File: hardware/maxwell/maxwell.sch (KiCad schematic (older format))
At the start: 34 parts, among them J1 Canbus 1, J2 Canbus 2, J3 Neopixel, J4 Boot Selection Jumper, J5 Charger Output, J6 Programmer, Q1 BSS138, U1 MCP2515-E/ST-SOIC, U2 SN65HVD233, U3 ITEAD_HC-05, U4 SIM800L_5-pin, U5 BOOST_BOARD, U6 TPS2511, Y1 16M

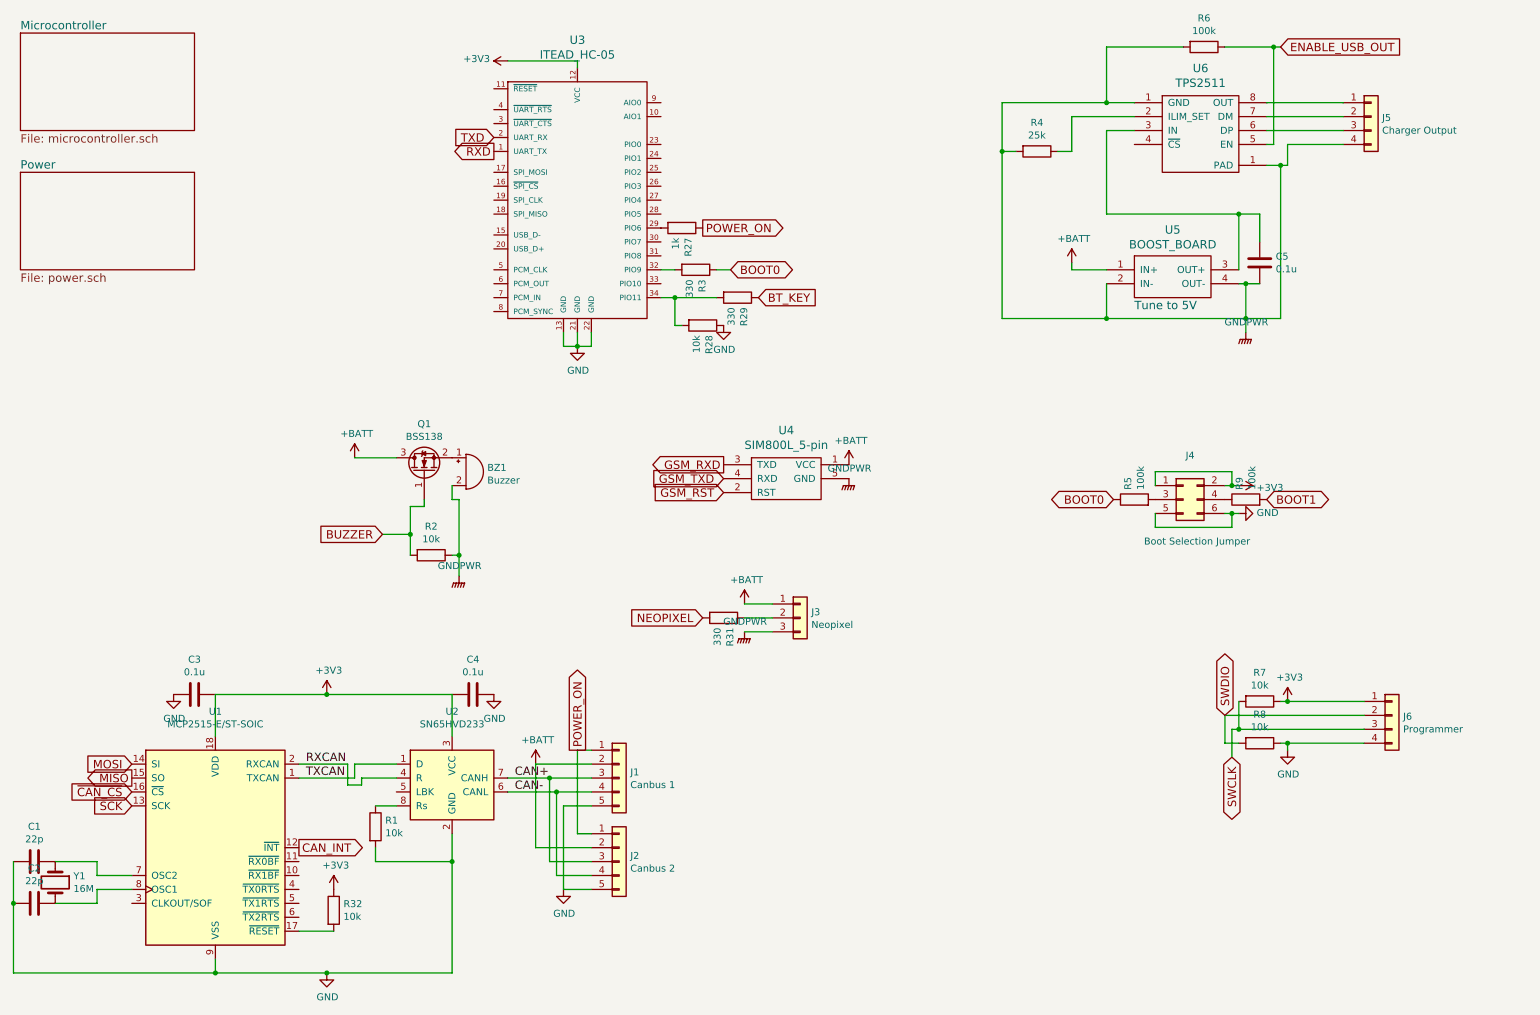
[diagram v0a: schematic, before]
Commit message: Fixed just...an unbelievable number of bugs.
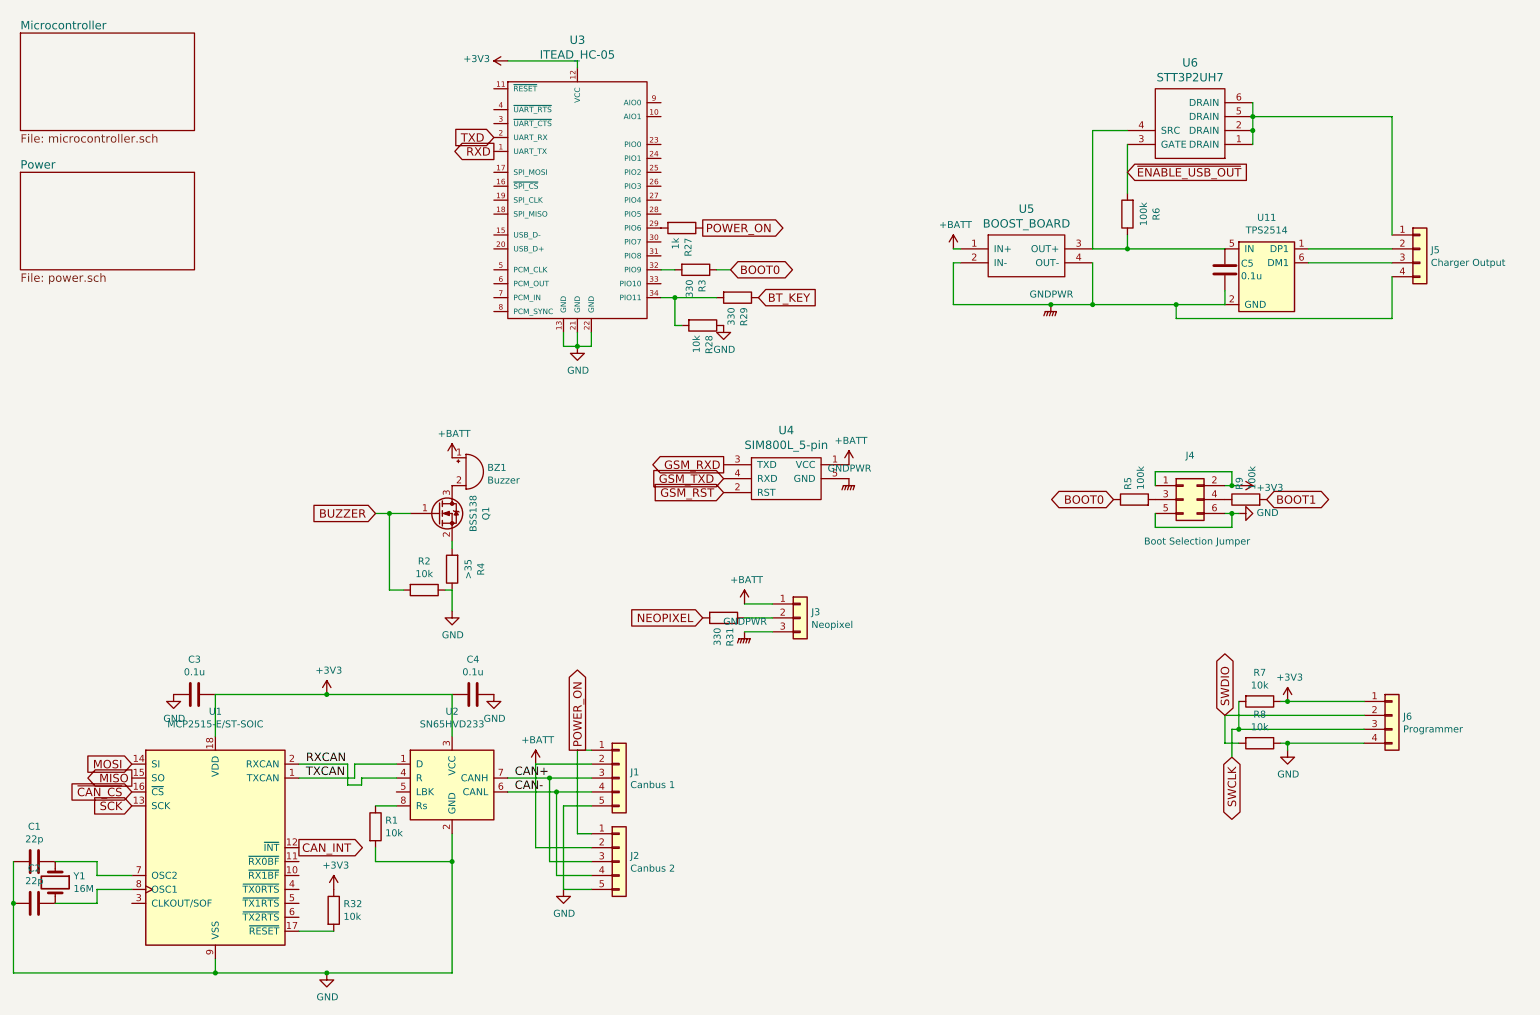
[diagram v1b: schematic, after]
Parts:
- removed U6: TPS2511, kicad-castellated-breakouts:SSOP8-1.27MM-CASTELLATED, symbol TPS2511
- added U11: TPS2514, adamgreig/agg-kicad/agg.pretty:SOT-23-6, symbol TPS2514
- added U6: STT3P2UH7, adamgreig/agg-kicad/agg.pretty:SOT-23-6, symbol STT3P2UH7
- R4: value 25k -> >35
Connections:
- net ENABLE_USB_OUT is gone; now on an unnamed net: R6.1
- net +BATT: now also BZ1.1 (-); no longer Q1.3 (D)
- net GND: now also R2.1, R4.1
- net GNDPWR: now also U11.2 (GND); no longer BZ1.2 (+), R2.1, R4.2, R6.2
- net at C5.1, U5.3 (OUT+): now also U11.5 (IN), U6.4 (SRC)
- net at J5.3 (Pin_3): now also U11.6 (DM1)
- net at J5.2 (Pin_2): now also U11.1 (DP1)
- net at J5.1 (Pin_1): now also U6.1 (DRAIN), U6.2 (DRAIN), U6.5 (DRAIN), U6.6 (DRAIN)
- net at Q1.2 (S): now also R4.2; no longer BZ1.1 (-)
- new net: BZ1.2 (+), Q1.3 (D)
- new net ~ENABLE_USB_OUT: R6.2, U6.3 (GATE)
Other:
- note removed: "Tune to 5V"
- moved on the sheet: C5, J5, Q1, R2, R6, U5
